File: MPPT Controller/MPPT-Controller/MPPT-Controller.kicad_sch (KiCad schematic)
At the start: 47 parts, among them J1 Conn_01x02_Pin, J2 Conn_01x02_Pin, J3 Conn_01x02_Pin, J4 Conn_01x02_Pin, Q1 IRL540N, SW1 SW_SPDT, U1 ADS1115IDGS, U4 LM1117DT-3.3, U5 LM2596S-ADJ, U6 TC4422

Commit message: Create ~MPPT-Controller.kicad_pcb.lck
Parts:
- SW1: footprint Button_Switch_SMD:SW_Push_1P1T_XKB_TS-1187A -> Connector_PinHeader_2.54mm:PinHeader_1x03_P2.54mm_Vertical
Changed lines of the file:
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@@
 			)
 		)
-		(property "Footprint" "Button_Switch_SMD:SW_Push_1P1T_XKB_TS-1187A"
+		(property "Footprint" "Connector_PinHeader_2.54mm:PinHeader_1x03_P2.54mm_Vertical"
 			(at 181.61 27.94 0)
 			(effects

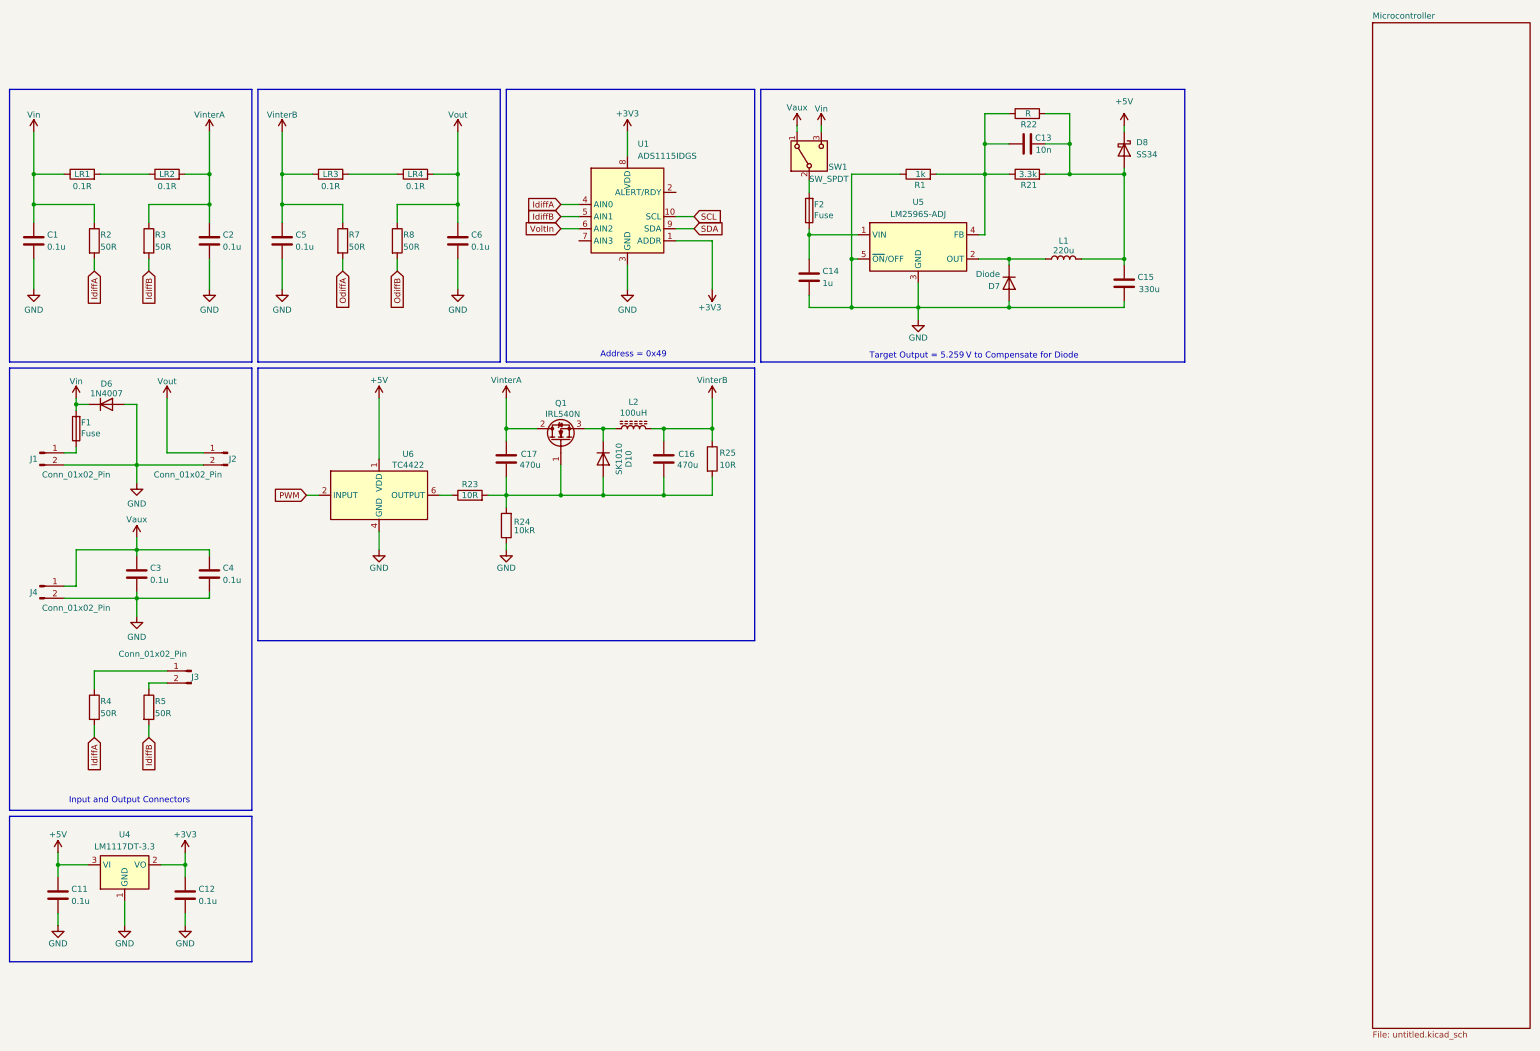
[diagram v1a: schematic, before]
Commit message: Add 2nd Power Measure
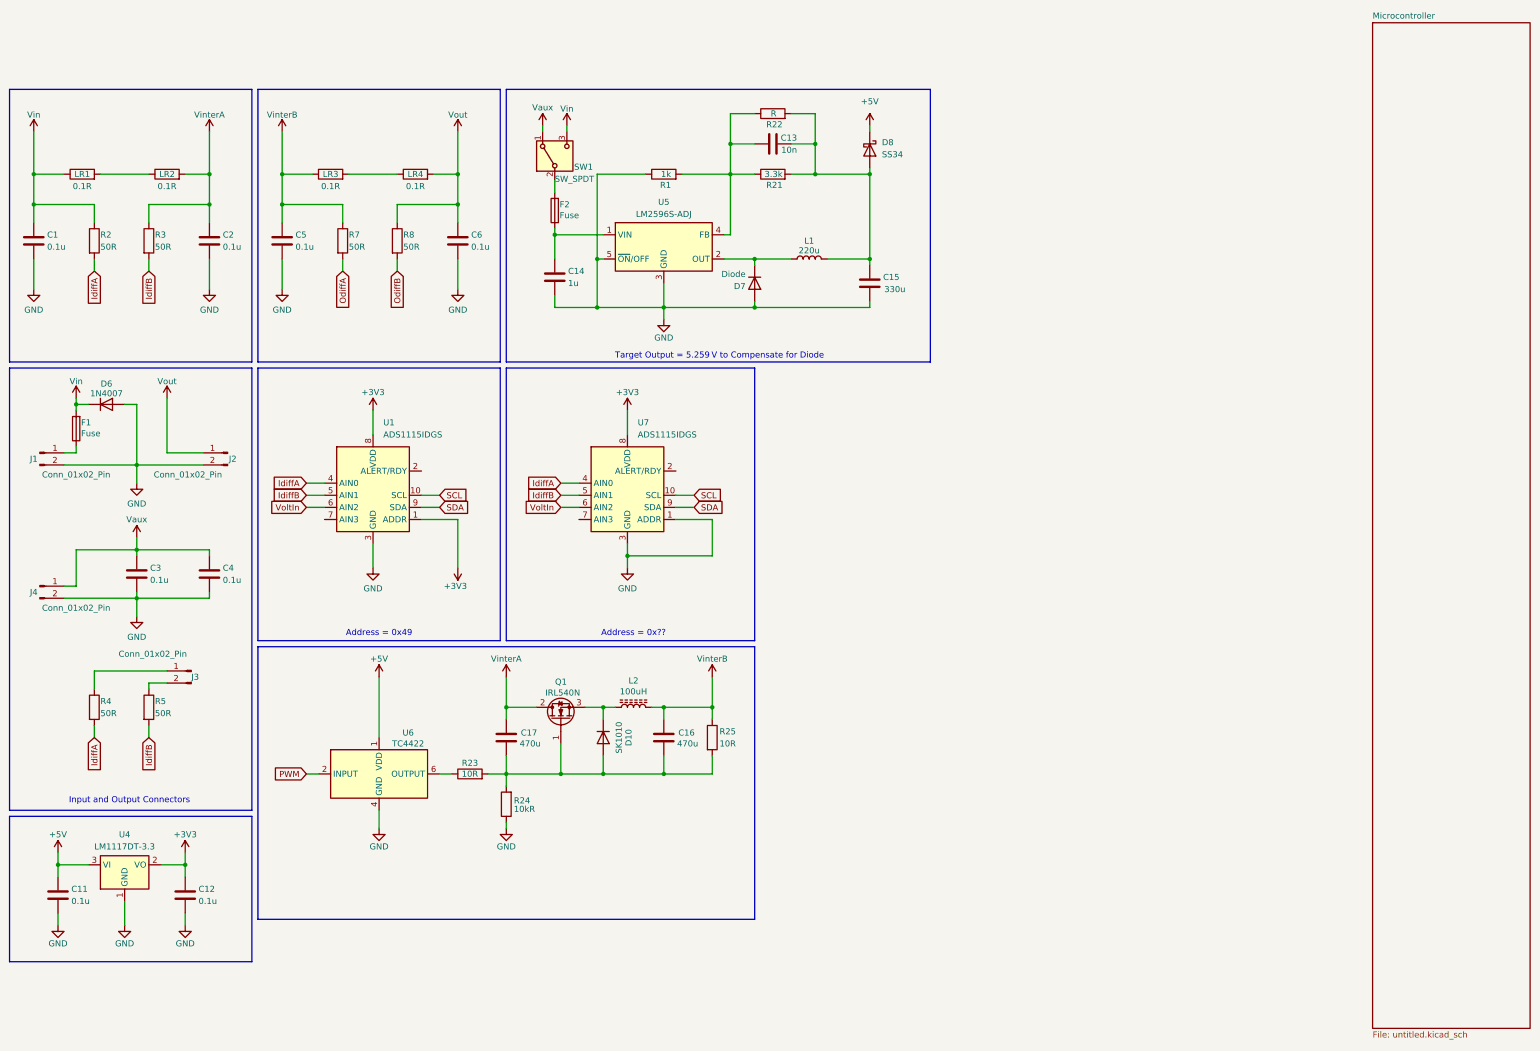
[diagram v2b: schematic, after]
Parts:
- added U7: ADS1115IDGS, Package_SO:TSSOP-10_3x3mm_P0.5mm, symbol Analog_ADC:ADS1115IDGS
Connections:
- net +3V3: now also U7.8 (VDD)
- net GND: now also U7.1 (ADDR), U7.3 (GND)
- net IdiffA: now also U7.4 (AIN0)
- net IdiffB: now also U7.5 (AIN1)
- net SCL: now also U7.10 (SCL)
- net SDA: now also U7.9 (SDA)
- net VoltIn: now also U7.6 (AIN2)
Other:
- note added: "Address = 0x??"
- moved on the sheet: C13, C14, C15, C16, C17, D10, D7, D8, F2, L1, L2, Q1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
